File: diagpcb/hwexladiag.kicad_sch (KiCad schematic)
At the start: 15 parts, among them J1 PINHEADER, Q1 2N7002, Q2 2N7002, SW1 SW_Push, U1 HC05, U2 HT7533-1

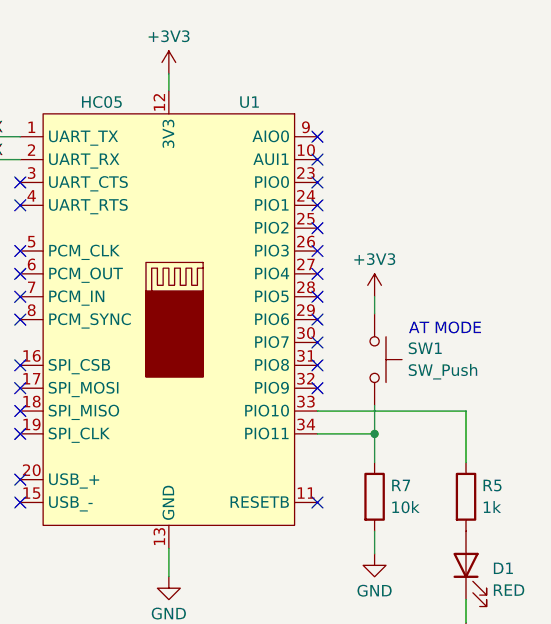
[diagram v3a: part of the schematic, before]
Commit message: diag: pin 31 for red LED.
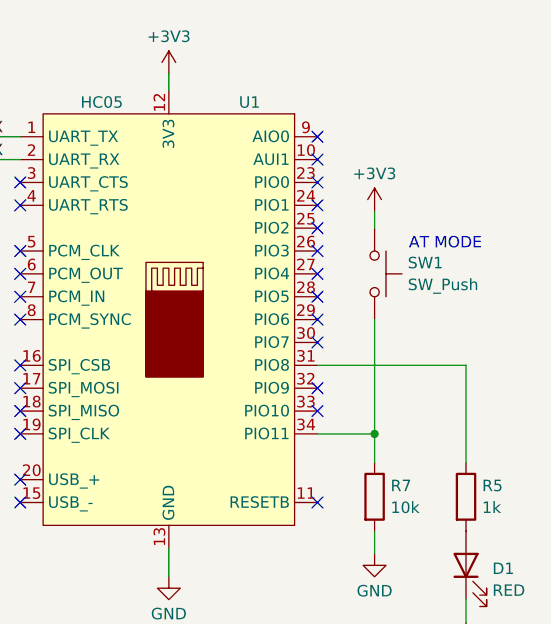
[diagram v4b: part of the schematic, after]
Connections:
- net at U1.31 (PIO8): now also R5.1
- net at U1.33 (PIO10): no longer R5.1
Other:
- moved on the sheet: SW1
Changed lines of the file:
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@@
   (no_connect (at 123.825 77.47))
   (no_connect (at 123.825 44.45))
-  (no_connect (at 156.845 62.23))
+  (no_connect (at 156.845 67.31))
   (no_connect (at 123.825 62.23))
   (wire (pts (xy 96.52 27.305) (xy 96.52 29.21))
@@
     (stroke (width 0) (type default))
   )
-  (wire (pts (xy 173.355 67.31) (xy 173.355 73.025))
+  (wire (pts (xy 173.355 62.23) (xy 173.355 73.025))
     (stroke (width 0) (type default))
   )
@@
     (stroke (width 0) (type default))
   )
-  (wire (pts (xy 163.195 54.61) (xy 163.195 56.515))
+  (wire (pts (xy 163.195 45.085) (xy 163.195 46.99))
     (stroke (width 0) (type default))
   )
@@
     (stroke (width 0) (type default))
   )
-  (wire (pts (xy 163.195 69.85) (xy 163.195 66.675))
-    (stroke (width 0) (type default))
-  )
-  (wire (pts (xy 156.845 67.31) (xy 173.355 67.31))
+  (wire (pts (xy 163.195 69.85) (xy 163.195 57.15))
+    (stroke (width 0) (type default))
+  )
+  (wire (pts (xy 156.845 62.23) (xy 173.355 62.23))
     (stroke (width 0) (type default))
   )
@@
     (stroke (width 0) (type default))
   )
-  (text "AT MODE" (at 167.005 59.055 0)
+  (text "AT MODE" (at 167.005 49.53 0)
     (effects (font (size 1.27 1.27)) (justify left bottom))
   )
@@
     )
   )
-  (symbol (lib_id "power:+3V3") (at 163.195 54.61 0) (unit 1)
-    (in_bom yes) (on_board yes) (dnp no) (fields_autoplaced)
-    (property "Reference" "#PWR010" (at 163.195 58.42 0)
-      (effects (font (size 1.27 1.27)) hide)
-    )
-    (property "Value" "+3V3" (at 163.195 50.4769 0)
-      (effects (font (size 1.27 1.27)))
-    )
-    (property "Footprint" "" (at 163.195 54.61 0)
-      (effects (font (size 1.27 1.27)) hide)
-    )
-    (property "Datasheet" "" (at 163.195 54.61 0)
+  (symbol (lib_id "power:+3V3") (at 163.195 45.085 0) (unit 1)
+    (in_bom yes) (on_board yes) (dnp no) (fields_autoplaced)
+    (property "Reference" "#PWR010" (at 163.195 48.895 0)
+      (effects (font (size 1.27 1.27)) hide)
+    )
+    (property "Value" "+3V3" (at 163.195 40.9519 0)
+      (effects (font (size 1.27 1.27)))
+    )
+    (property "Footprint" "" (at 163.195 45.085 0)
+      (effects (font (size 1.27 1.27)) hide)
+    )
+    (property "Datasheet" "" (at 163.195 45.085 0)
       (effects (font (size 1.27 1.27)) hide)
     )
@@
     )
   )
-  (symbol (lib_id "Switch:SW_Push") (at 163.195 61.595 270) (unit 1)
-    (in_bom yes) (on_board yes) (dnp no) (fields_autoplaced)
-    (property "Reference" "SW1" (at 166.878 60.3829 90)
-      (effects (font (size 1.27 1.27)) (justify left))
-    )
-    (property "Value" "SW_Push" (at 166.878 62.8071 90)
-      (effects (font (size 1.27 1.27)) (justify left))
-    )
-    (property "Footprint" "Button_Switch_SMD:SW_SPST_EVQPE1" (at 168.275 61.595 0)
-      (effects (font (size 1.27 1.27)) hide)
-    )
-    (property "Datasheet" "~" (at 168.275 61.595 0)
-      (effects (font (size 1.27 1.27)) hide)
-    )
+  (symbol (lib_id "Switch:SW_Push") (at 163.195 52.07 270) (unit 1)
+    (in_bom yes) (on_board yes) (dnp no) (fields_autoplaced)
+    (property "Reference" "SW1" (at 166.878 50.8579 90)
+      (effects (font (size 1.27 1.27)) (justify left))
+    )
+    (property "Value" "SW_Push" (at 166.878 53.2821 90)
+      (effects (font (size 1.27 1.27)) (justify left))
+    )
+    (property "Footprint" "Button_Switch_SMD:SW_SPST_EVQPE1" (at 168.275 52.07 0)
+      (effects (font (size 1.27 1.27)) hide)
+    )
+    (property "Datasheet" "~" (at 168.275 52.07 0)
+      (effects (font (size 1.27 1.27)) hide)
+    )

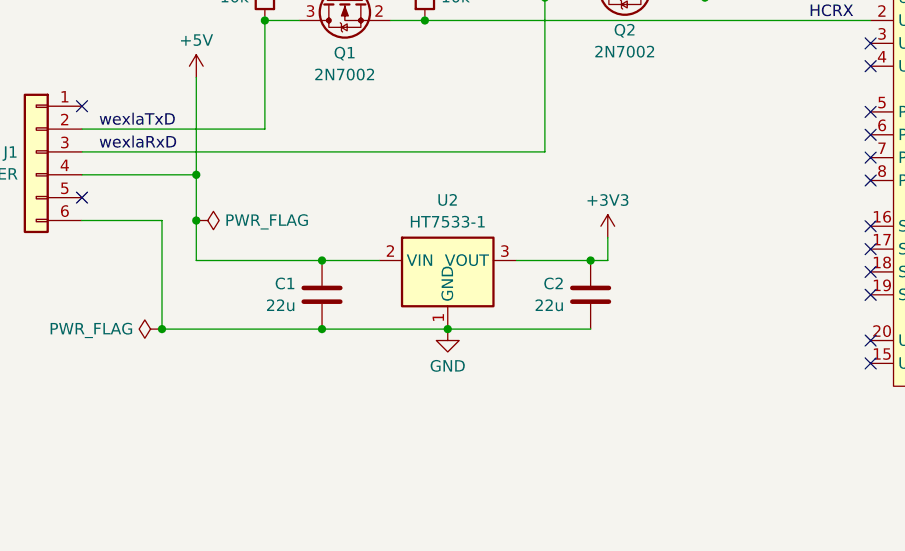
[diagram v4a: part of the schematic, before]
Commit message: diag: use input resistor 10R.
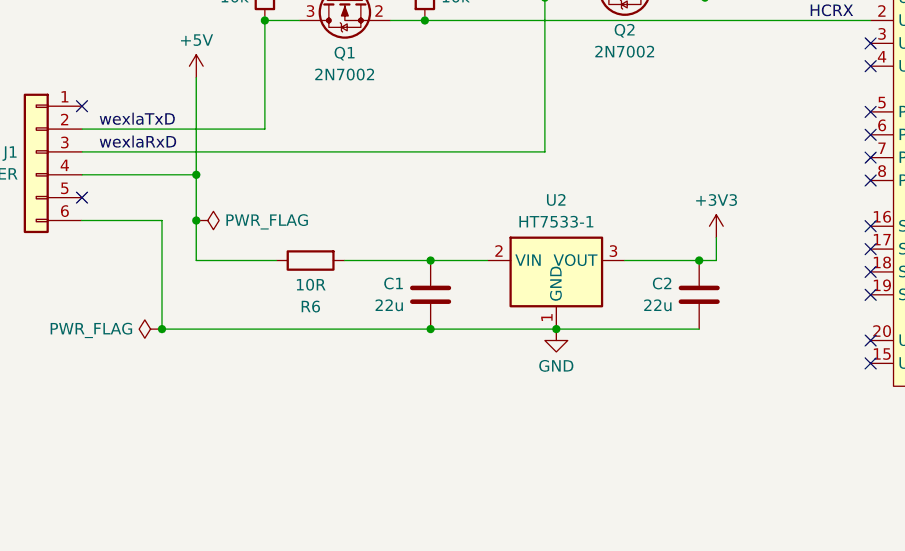
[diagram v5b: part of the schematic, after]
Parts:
- added R6: 10R, Resistor_SMD:R_0805_2012Metric, symbol Device:R
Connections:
- net +5V: now also R6.1; no longer C1.1, U2.2 (VIN)
- new net: C1.1, R6.2, U2.2 (VIN)
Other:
- moved on the sheet: C1, C2, U2
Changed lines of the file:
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@@
   (junction (at 48.895 61.595) (diameter 0) (color 0 0 0 0)
   )
-  (junction (at 62.865 66.04) (diameter 0) (color 0 0 0 0)
+  (junction (at 74.93 66.04) (diameter 0) (color 0 0 0 0)
   )
   (junction (at 65.405 29.845) (diameter 0) (color 0 0 0 0)
@@
   (junction (at 96.52 27.305) (diameter 0) (color 0 0 0 0)
   )
-  (junction (at 92.71 66.04) (diameter 0) (color 0 0 0 0)
+  (junction (at 104.775 66.04) (diameter 0) (color 0 0 0 0)
   )
   (junction (at 105.41 36.83) (diameter 0) (color 0 0 0 0)
@@
   (junction (at 48.895 56.515) (diameter 0) (color 0 0 0 0)
   )
-  (junction (at 62.865 73.66) (diameter 0) (color 0 0 0 0)
+  (junction (at 74.93 73.66) (diameter 0) (color 0 0 0 0)
   )
   (junction (at 163.195 69.85) (diameter 0) (color 0 0 0 0)
@@
   (junction (at 56.515 39.37) (diameter 0) (color 0 0 0 0)
   )
-  (junction (at 76.835 73.66) (diameter 0) (color 0 0 0 0)
+  (junction (at 88.9 73.66) (diameter 0) (color 0 0 0 0)
   )
   (no_connect (at 156.845 59.69))
@@
     (stroke (width 0) (type default))
   )
-  (wire (pts (xy 62.865 73.66) (xy 76.835 73.66))
+  (wire (pts (xy 74.93 73.66) (xy 88.9 73.66))
     (stroke (width 0) (type default))
   )
@@
     (stroke (width 0) (type default))
   )
-  (wire (pts (xy 76.835 73.66) (xy 92.71 73.66))
+  (wire (pts (xy 88.9 73.66) (xy 104.775 73.66))
     (stroke (width 0) (type default))
   )
@@
     (stroke (width 0) (type default))
   )
-  (wire (pts (xy 84.455 66.04) (xy 92.71 66.04))
+  (wire (pts (xy 96.52 66.04) (xy 104.775 66.04))
     (stroke (width 0) (type default))
   )
@@
     (stroke (width 0) (type default))
   )
-  (wire (pts (xy 92.71 66.04) (xy 94.615 66.04))
-    (stroke (width 0) (type default))
-  )
-  (wire (pts (xy 62.865 66.04) (xy 69.215 66.04))
+  (wire (pts (xy 104.775 66.04) (xy 106.68 66.04))
+    (stroke (width 0) (type default))
+  )
+  (wire (pts (xy 74.93 66.04) (xy 81.28 66.04))
     (stroke (width 0) (type default))
   )
@@
     (stroke (width 0) (type default))
   )
-  (wire (pts (xy 48.895 66.04) (xy 62.865 66.04))
+  (wire (pts (xy 48.895 66.04) (xy 57.785 66.04))
     (stroke (width 0) (type default))
   )
@@
     (stroke (width 0) (type default))
   )
-  (wire (pts (xy 94.615 63.5) (xy 94.615 66.04))
+  (wire (pts (xy 106.68 63.5) (xy 106.68 66.04))
     (stroke (width 0) (type default))
   )
@@
     (stroke (width 0) (type default))
   )
-  (wire (pts (xy 45.085 73.66) (xy 62.865 73.66))
+  (wire (pts (xy 45.085 73.66) (xy 74.93 73.66))
+    (stroke (width 0) (type default))
+  )
+  (wire (pts (xy 65.405 66.04) (xy 74.93 66.04))
     (stroke (width 0) (type default))
   )
@@
     )
   )
-  (symbol (lib_id "Regulator_Linear:HT75xx-1-SOT89") (at 76.835 68.58 0) (unit 1)
+  (symbol (lib_id "Regulator_Linear:HT75xx-1-SOT89") (at 88.9 68.58 0) (unit 1)
     (in_bom yes) (on_board yes) (dnp no)
-    (property "Reference" "U2" (at 76.835 59.3557 0)
-      (effects (font (size 1.27 1.27)))
-    )
-    (property "Value" "HT7533-1" (at 76.835 61.7799 0)
-      (effects (font (size 1.27 1.27)))
-    )
-    (property "Footprint" "Package_TO_SOT_SMD:SOT-89-3" (at 76.835 60.325 0)
+    (property "Reference" "U2" (at 88.9 59.3557 0)
+      (effects (font (size 1.27 1.27)))
+    )
+    (property "Value" "HT7533-1" (at 88.9 61.7799 0)
+      (effects (font (size 1.27 1.27)))
+    )
+    (property "Footprint" "Package_TO_SOT_SMD:SOT-89-3" (at 88.9 60.325 0)
       (effects (font (size 1.27 1.27) italic) hide)
     )
-    (property "Datasheet" "https://www.holtek.com/documents/10179/116711/HT75xx-1v250.pdf" (at 76.835 66.04 0)
+    (property "Datasheet" "https://www.holtek.com/documents/10179/116711/HT75xx-1v250.pdf" (at 88.9 66.04 0)
       (effects (font (size 1.27 1.27)) hide)
     )
@@
     )
   )
-  (symbol (lib_id "power:GND") (at 76.835 73.66 0) (mirror y) (unit 1)
-    (in_bom yes) (on_board yes) (dnp no) (fields_autoplaced)
-    (property "Reference" "#PWR04" (at 76.835 80.01 0)
-      (effects (font (size 1.27 1.27)) hide)
-    )
-    (property "Value" "GND" (at 76.835 77.7931 0)
-      (effects (font (size 1.27 1.27)))
-    )
-    (property "Footprint" "" (at 76.835 73.66 0)
-      (effects (font (size 1.27 1.27)) hide)
-    )
-    (property "Datasheet" "" (at 76.835 73.66 0)
+  (symbol (lib_id "Device:R") (at 61.595 66.04 90) (mirror x) (unit 1)
+    (in_bom yes) (on_board yes) (dnp no)
+    (property "Reference" "R6" (at 61.595 71.2003 90)
+      (effects (font (size 1.27 1.27)))
+    )
+    (property "Value" "10R" (at 61.595 68.7761 90)
+      (effects (font (size 1.27 1.27)))
+    )
+    (property "Footprint" "Resistor_SMD:R_0805_2012Metric" (at 61.595 64.262 90)
+      (effects (font (size 1.27 1.27)) hide)
+    )
+    (property "Datasheet" "~" (at 61.595 66.04 0)
+      (effects (font (size 1.27 1.27)) hide)
+    )
+    (pin "1")
+    (pin "2")
+    (instances
+      (project "hwexladiag"
+        (path "/41af901d-6d9d-4dc3-adca-d33b9d619d2e"
+          (reference "R6") (unit 1)
+        )
+      )
+    )
+  )
+  (symbol (lib_id "power:GND") (at 88.9 73.66 0) (mirror y) (unit 1)
+    (in_bom yes) (on_board yes) (dnp no) (fields_autoplaced)
+    (property "Reference" "#PWR04" (at 88.9 80.01 0)
+      (effects (font (size 1.27 1.27)) hide)
+    )
+    (property "Value" "GND" (at 88.9 77.7931 0)
+      (effects (font (size 1.27 1.27)))
+    )
+    (property "Footprint" "" (at 88.9 73.66 0)
+      (effects (font (size 1.27 1.27)) hide)
+    )
+    (property "Datasheet" "" (at 88.9 73.66 0)
       (effects (font (size 1.27 1.27)) hide)
     )
@@
     )
   )
-  (symbol (lib_id "Device:C") (at 92.71 69.85 0) (mirror y) (unit 1)
-    (in_bom yes) (on_board yes) (dnp no) (fields_autoplaced)
-    (property "Reference" "C2" (at 89.789 68.6379 0)
-      (effects (font (size 1.27 1.27)) (justify left))
-    )
-    (property "Value" "22u" (at 89.789 71.0621 0)
-      (effects (font (size 1.27 1.27)) (justify left))
-    )
-    (property "Footprint" "Capacitor_SMD:C_0805_2012Metric" (at 91.7448 73.66 0)
-      (effects (font (size 1.27 1.27)) hide)
-    )
-    (property "Datasheet" "~" (at 92.71 69.85 0)
+  (symbol (lib_id "Device:C") (at 104.775 69.85 0) (mirror y) (unit 1)
+    (in_bom yes) (on_board yes) (dnp no) (fields_autoplaced)
+    (property "Reference" "C2" (at 101.854 68.6379 0)
+      (effects (font (size 1.27 1.27)) (justify left))
+    )
+    (property "Value" "22u" (at 101.854 71.0621 0)
+      (effects (font (size 1.27 1.27)) (justify left))
+    )
+    (property "Footprint" "Capacitor_SMD:C_0805_2012Metric" (at 103.8098 73.66 0)
+      (effects (font (size 1.27 1.27)) hide)
+    )
+    (property "Datasheet" "~" (at 104.775 69.85 0)
       (effects (font (size 1.27 1.27)) hide)
     )
@@
     )
   )
-  (symbol (lib_id "power:+3V3") (at 94.615 63.5 0) (unit 1)
-    (in_bom yes) (on_board yes) (dnp no) (fields_autoplaced)
-    (property "Reference" "#PWR05" (at 94.615 67.31 0)
-      (effects (font (size 1.27 1.27)) hide)
-    )
-    (property "Value" "+3V3" (at 94.615 59.3669 0)
-      (effects (font (size 1.27 1.27)))
-    )
-    (property "Footprint" "" (at 94.615 63.5 0)
-      (effects (font (size 1.27 1.27)) hide)
-    )
-    (property "Datasheet" "" (at 94.615 63.5 0)
+  (symbol (lib_id "power:+3V3") (at 106.68 63.5 0) (unit 1)
+    (in_bom yes) (on_board yes) (dnp no) (fields_autoplaced)
+    (property "Reference" "#PWR05" (at 106.68 67.31 0)
+      (effects (font (size 1.27 1.27)) hide)
+    )
+    (property "Value" "+3V3" (at 106.68 59.3669 0)
+      (effects (font (size 1.27 1.27)))
+    )
+    (property "Footprint" "" (at 106.68 63.5 0)
+      (effects (font (size 1.27 1.27)) hide)
+    )
+    (property "Datasheet" "" (at 106.68 63.5 0)
       (effects (font (size 1.27 1.27)) hide)
     )
@@
     )
   )
-  (symbol (lib_id "Device:C") (at 62.865 69.85 0) (mirror y) (unit 1)
-    (in_bom yes) (on_board yes) (dnp no) (fields_autoplaced)
-    (property "Reference" "C1" (at 59.944 68.6379 0)
-      (effects (font (size 1.27 1.27)) (justify left))
-    )
-    (property "Value" "22u" (at 59.944 71.0621 0)
-      (effects (font (size 1.27 1.27)) (justify left))
-    )
-    (property "Footprint" "Capacitor_SMD:C_0805_2012Metric" (at 61.8998 73.66 0)
-      (effects (font (size 1.27 1.27)) hide)
-    )
-    (property "Datasheet" "~" (at 62.865 69.85 0)
-      (effects (font (size 1.27 1.27)) hide)
-    )
+  (symbol (lib_id "Device:C") (at 74.93 69.85 0) (mirror y) (unit 1)
+    (in_bom yes) (on_board yes) (dnp no) (fields_autoplaced)
+    (property "Reference" "C1" (at 72.009 68.6379 0)
+      (effects (font (size 1.27 1.27)) (justify left))
+    )
+    (property "Value" "22u" (at 72.009 71.0621 0)
+      (effects (font (size 1.27 1.27)) (justify left))
+    )
+    (property "Footprint" "Capacitor_SMD:C_0805_2012Metric" (at 73.9648 73.66 0)
+      (effects (font (size 1.27 1.27)) hide)
+    )
+    (property "Datasheet" "~" (at 74.93 69.85 0)
+      (effects (font (size 1.27 1.27)) hide)
+    )

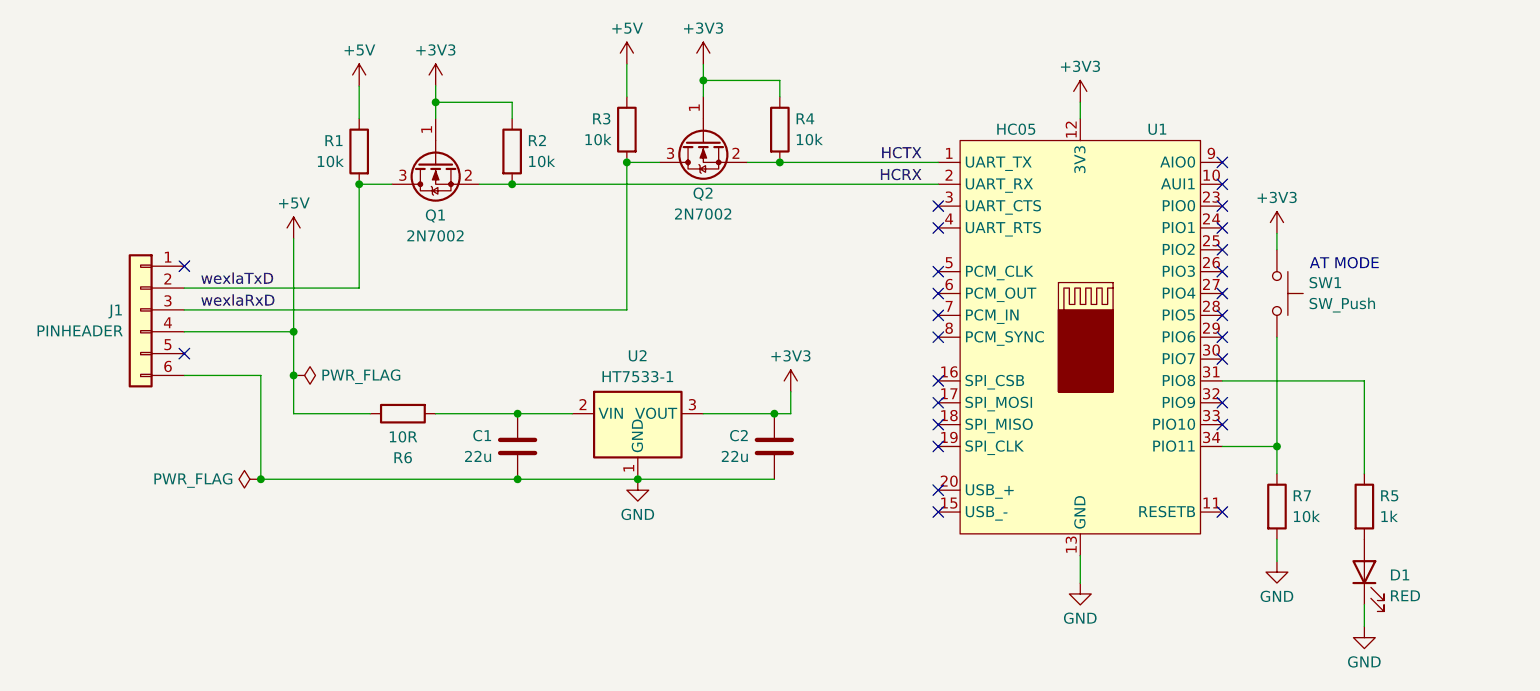
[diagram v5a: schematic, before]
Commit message: Add jumper for AT pin external connection.
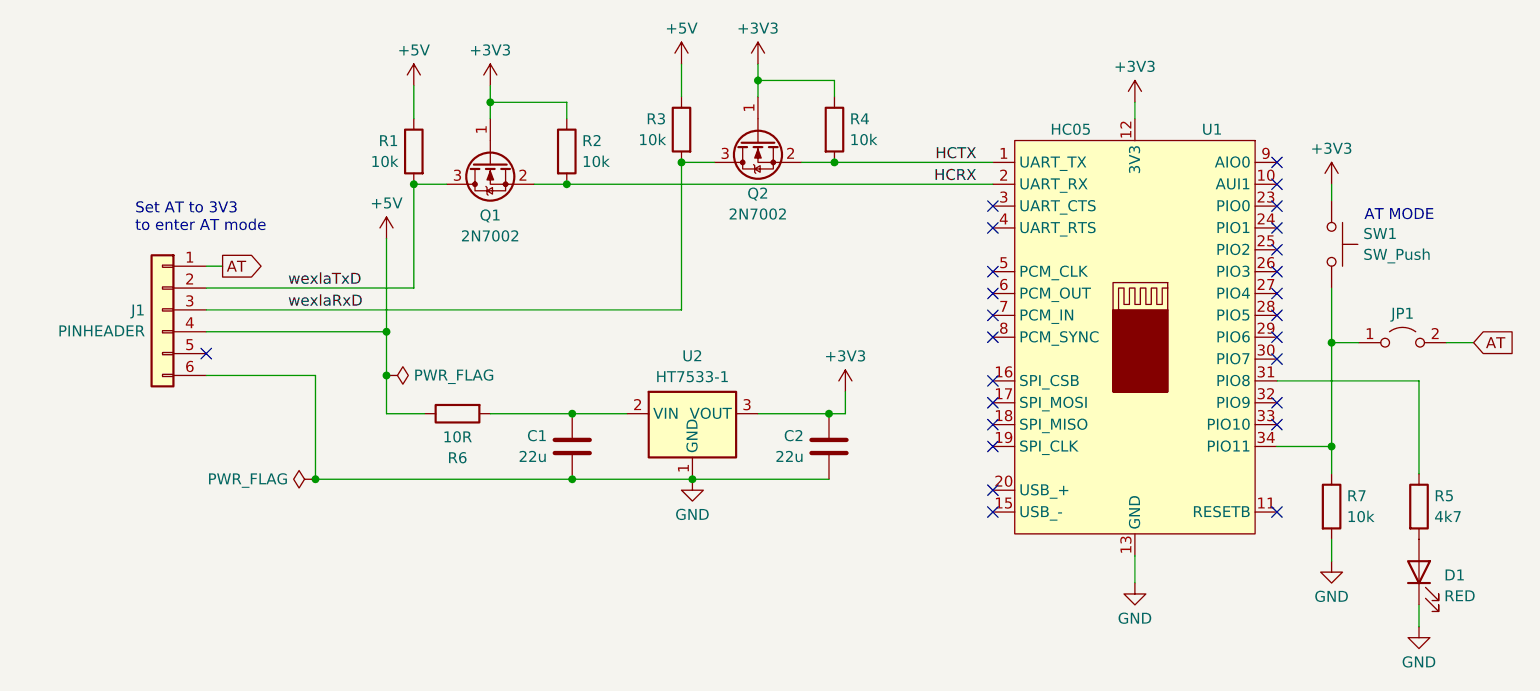
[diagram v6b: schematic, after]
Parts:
- added JP1: ~, Jumper:SolderJumper-2_P1.3mm_Open_RoundedPad1.0x1.5mm, symbol Jumper:Jumper_2_Open
- R5: value 1k -> 4k7
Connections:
- net AT: now reaches J1.1 (Pin_1)
- net AT: now also JP1.2 (B)
- net at R7.1, SW1.2, U1.34 (PIO11): now also JP1.1 (A)
- no-connect marks 27 -> 26
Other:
- note added: "Set AT to 3V3 to enter AT mode"
- moved on the sheet: C1, C2, D1, J1, Q1, Q2, R1, R2, R3, R4, R5, R6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
